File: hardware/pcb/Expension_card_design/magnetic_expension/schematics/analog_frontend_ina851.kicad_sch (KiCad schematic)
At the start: 36 parts, among them U5 INA851RGTR, U6 INA851RGTR, U7 INA851RGTR

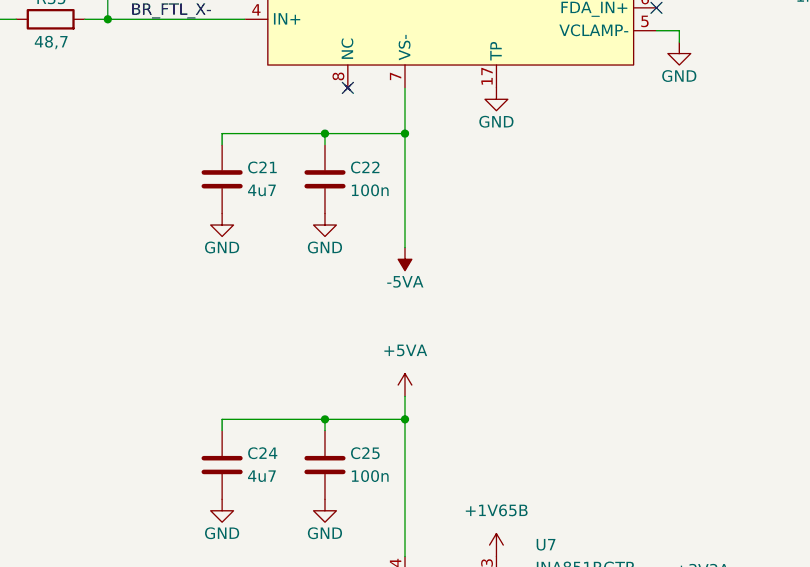
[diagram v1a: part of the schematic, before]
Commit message: Work in progress rev2
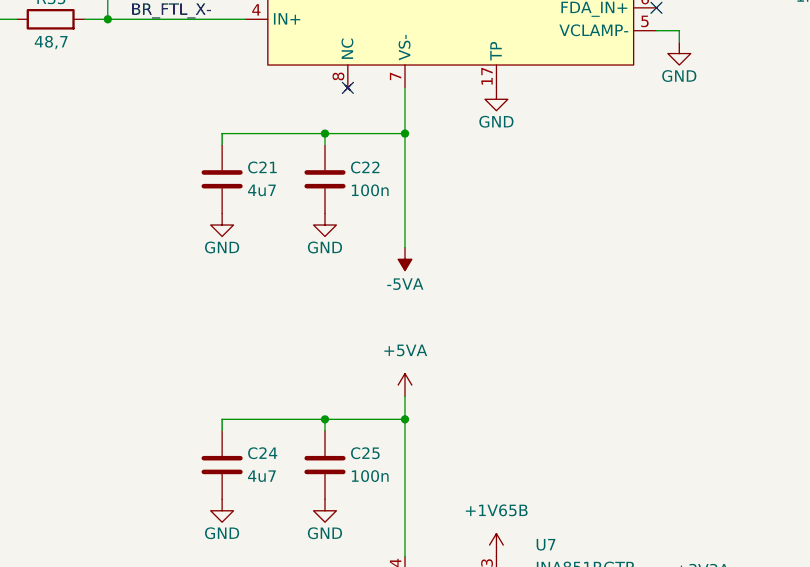
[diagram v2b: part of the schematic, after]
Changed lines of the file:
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@@
 		)
 		(property "Value" "-5VA"
-			(at 81.28 101.6 0)
+			(at 81.28 101.854 0)
 			(effects
 				(font
